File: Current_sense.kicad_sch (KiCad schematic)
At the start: 5 parts, among them U33 INA180A4

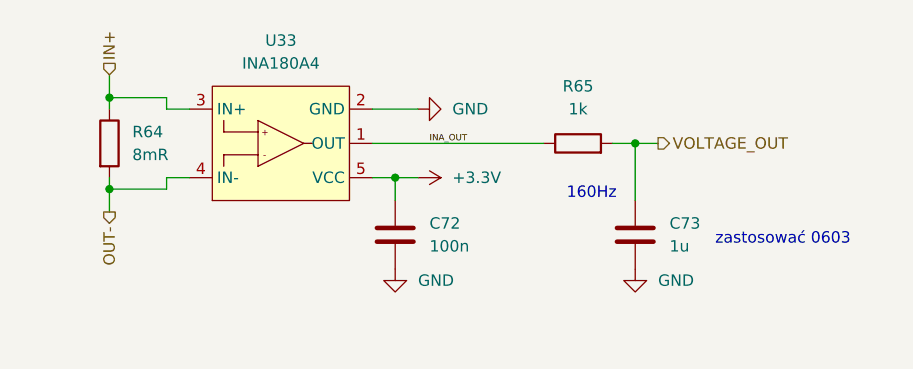
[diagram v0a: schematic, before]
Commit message: start design power input
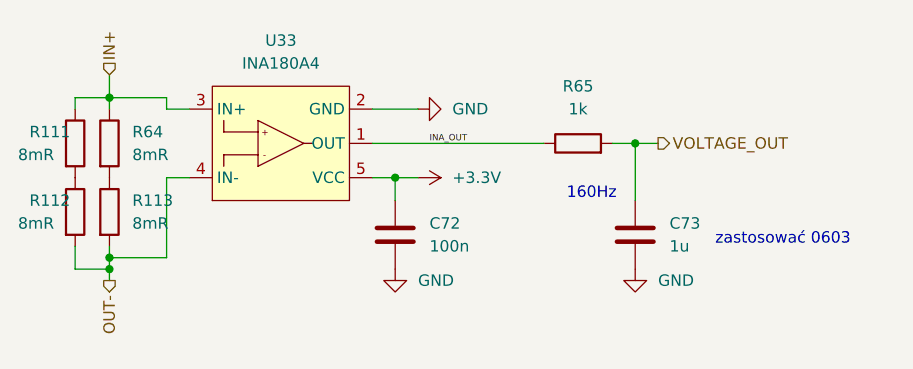
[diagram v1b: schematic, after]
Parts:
- added R111, R112, R113: 8mR, Resistor_SMD:R_2512_6332Metric_Pad1.40x3.35mm_HandSolder, symbol Device:R
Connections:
- net IN+: now also R111.1
- net OUT-: now also R112.2, R113.2; no longer R64.2
- new net: R111.2, R112.1
- new net: R113.1, R64.2
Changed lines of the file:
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@@
   (junction (at 104.14 77.47) (diameter 0) (color 0 0 0 0)
   )
-  (junction (at 104.14 87.63) (diameter 0) (color 0 0 0 0)
+  (junction (at 104.14 95.25) (diameter 0) (color 0 0 0 0)
+  )
+  (junction (at 104.14 96.52) (diameter 0) (color 0 0 0 0)
   )
   (wire (pts (xy 110.49 77.47) (xy 110.49 78.74))
     (stroke (width 0) (type default) (color 0 0 0 0))
   )
-  (wire (pts (xy 104.14 87.63) (xy 110.49 87.63))
-    (stroke (width 0) (type default) (color 0 0 0 0))
-  )
   (wire (pts (xy 162.56 82.55) (xy 165.1 82.55))
     (stroke (width 0) (type default) (color 0 0 0 0))
   )
-  (wire (pts (xy 104.14 87.63) (xy 104.14 90.17))
-    (stroke (width 0) (type default) (color 0 0 0 0))
-  )
   (wire (pts (xy 104.14 78.74) (xy 104.14 77.47))
     (stroke (width 0) (type default) (color 0 0 0 0))
@@
     (stroke (width 0) (type default) (color 0 0 0 0))
   )
+  (wire (pts (xy 110.49 95.25) (xy 104.14 95.25))
+    (stroke (width 0) (type default) (color 0 0 0 0))
+  )
+  (wire (pts (xy 100.33 77.47) (xy 104.14 77.47))
+    (stroke (width 0) (type default) (color 0 0 0 0))
+  )
   (wire (pts (xy 104.14 74.93) (xy 104.14 77.47))
     (stroke (width 0) (type default) (color 0 0 0 0))
   )
-  (wire (pts (xy 104.14 86.36) (xy 104.14 87.63))
+  (wire (pts (xy 104.14 96.52) (xy 104.14 97.79))
+    (stroke (width 0) (type default) (color 0 0 0 0))
+  )
+  (wire (pts (xy 100.33 96.52) (xy 104.14 96.52))
+    (stroke (width 0) (type default) (color 0 0 0 0))
+  )
+  (wire (pts (xy 100.33 78.74) (xy 100.33 77.47))
     (stroke (width 0) (type default) (color 0 0 0 0))
   )
@@
     (stroke (width 0) (type default) (color 0 0 0 0))
   )
-  (wire (pts (xy 110.49 87.63) (xy 110.49 86.36))
+  (wire (pts (xy 104.14 93.98) (xy 104.14 95.25))
+    (stroke (width 0) (type default) (color 0 0 0 0))
+  )
+  (wire (pts (xy 110.49 86.36) (xy 110.49 95.25))
     (stroke (width 0) (type default) (color 0 0 0 0))
   )
@@
     (stroke (width 0) (type default) (color 0 0 0 0))
   )
+  (wire (pts (xy 104.14 95.25) (xy 104.14 96.52))
+    (stroke (width 0) (type default) (color 0 0 0 0))
+  )
   (wire (pts (xy 133.35 82.55) (xy 152.4 82.55))
     (stroke (width 0) (type default) (color 0 0 0 0))
@@
   )
   (wire (pts (xy 110.49 86.36) (xy 113.03 86.36))
+    (stroke (width 0) (type default) (color 0 0 0 0))
+  )
+  (wire (pts (xy 100.33 93.98) (xy 100.33 96.52))
     (stroke (width 0) (type default) (color 0 0 0 0))
   )
@@
     (effects (font (size 0.7 0.7)) (justify left bottom))
   )
-  (hierarchical_label "OUT-" (shape output) (at 104.14 90.17 270)
+  (hierarchical_label "OUT-" (shape output) (at 104.14 97.79 270)
     (effects (font (size 1.27 1.27)) (justify right))
   )
@@
     )
     (property "Datasheet" "~" (id 3) (at 162.56 92.71 0)
+      (effects (font (size 1.27 1.27)) hide)
+    )
+    (pin "1")
+    (pin "2")
+  )
+  (symbol (lib_id "Device:R") (at 100.33 90.17 0) (unit 1)
+    (in_bom yes) (on_board yes)
+    (property "Reference" "R112" (id 0) (at 95.25 88.9 0)
+      (effects (font (size 1.27 1.27)) (justify left))
+    )
+    (property "Value" "8mR" (id 1) (at 93.98 91.44 0)
+      (effects (font (size 1.27 1.27)) (justify left))
+    )
+    (property "Footprint" "Resistor_SMD:R_2512_6332Metric_Pad1.40x3.35mm_HandSolder" (id 2) (at 98.552 90.17 90)
+      (effects (font (size 1.27 1.27)) hide)
+    )
+    (property "Datasheet" "~" (id 3) (at 100.33 90.17 0)
       (effects (font (size 1.27 1.27)) hide)
     )
@@
     (pin "1")
   )
+  (symbol (lib_id "Device:R") (at 104.14 90.17 0) (unit 1)
+    (in_bom yes) (on_board yes) (fields_autoplaced)
+    (property "Reference" "R113" (id 0) (at 106.68 88.8999 0)
+      (effects (font (size 1.27 1.27)) (justify left))
+    )
+    (property "Value" "8mR" (id 1) (at 106.68 91.4399 0)
+      (effects (font (size 1.27 1.27)) (justify left))
+    )
+    (property "Footprint" "Resistor_SMD:R_2512_6332Metric_Pad1.40x3.35mm_HandSolder" (id 2) (at 102.362 90.17 90)
+      (effects (font (size 1.27 1.27)) hide)
+    )
+    (property "Datasheet" "~" (id 3) (at 104.14 90.17 0)
+      (effects (font (size 1.27 1.27)) hide)
+    )
+    (pin "1")
+    (pin "2")
+  )
   (symbol (lib_id "Device:R") (at 156.21 82.55 90) (unit 1)
     (in_bom yes) (on_board yes) (fields_autoplaced)
@@
     (pin "1")
   )
+  (symbol (lib_id "Device:R") (at 100.33 82.55 0) (unit 1)
+    (in_bom yes) (on_board yes)
+    (property "Reference" "R111" (id 0) (at 95.25 81.28 0)
+      (effects (font (size 1.27 1.27)) (justify left))
+    )
+    (property "Value" "8mR" (id 1) (at 93.98 83.82 0)
+      (effects (font (size 1.27 1.27)) (justify left))
+    )
+    (property "Footprint" "Resistor_SMD:R_2512_6332Metric_Pad1.40x3.35mm_HandSolder" (id 2) (at 98.552 82.55 90)
+      (effects (font (size 1.27 1.27)) hide)
+    )
+    (property "Datasheet" "~" (id 3) (at 100.33 82.55 0)
+      (effects (font (size 1.27 1.27)) hide)
+    )
+    (pin "1")
+    (pin "2")
+  )
   (symbol (lib_id "Device:C") (at 135.89 92.71 0) (unit 1)
